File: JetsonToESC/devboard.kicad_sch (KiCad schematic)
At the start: 9 parts, among them U1 ESP32-C3_SUPERMINI_TH, U4 MCP23018x-x-SS

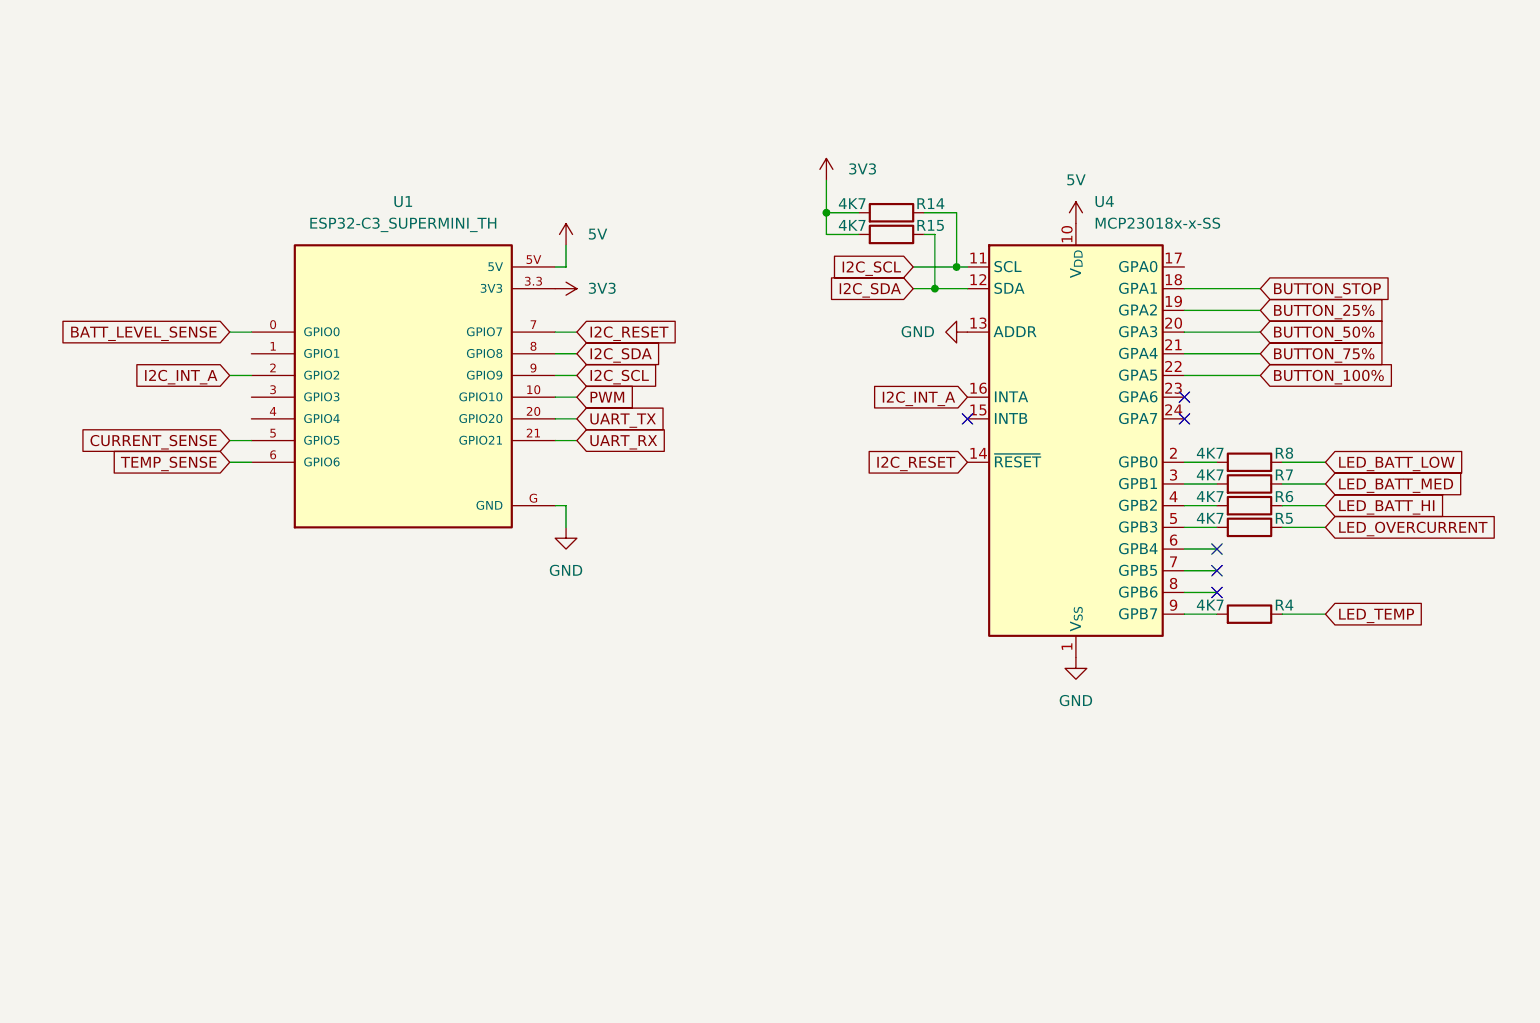
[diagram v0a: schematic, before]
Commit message: Design and routing done
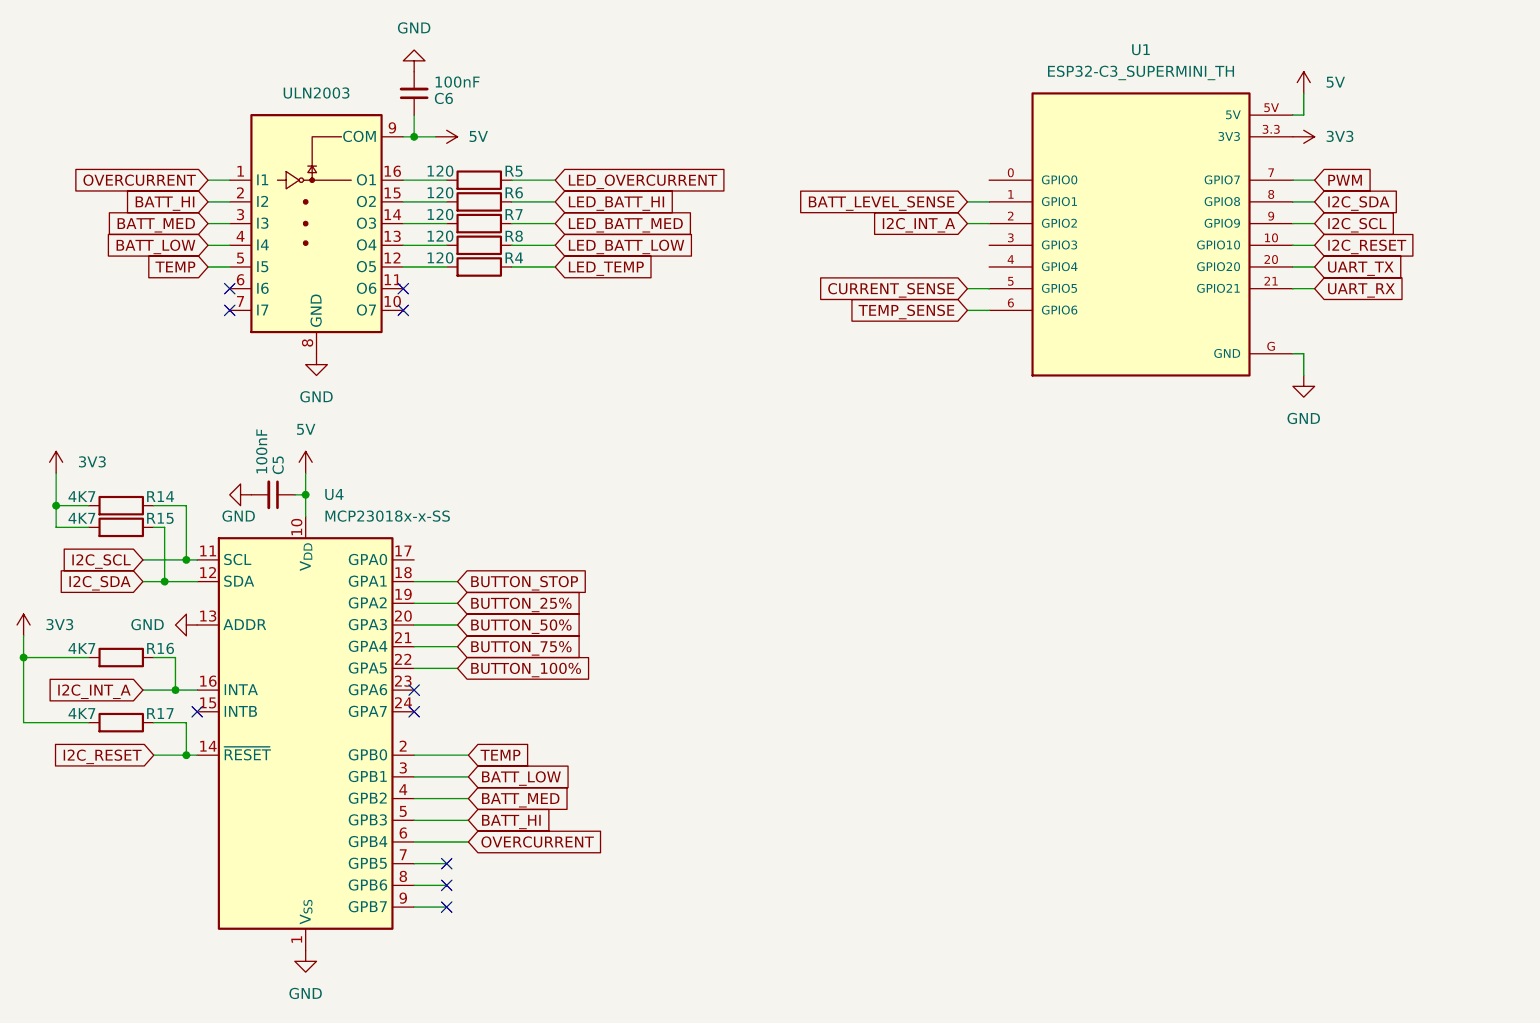
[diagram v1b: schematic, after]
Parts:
- added C5, C6: 100nF, Capacitor_SMD:C_0603_1608Metric, symbol Device:C_Small
- added R16, R17: 4K7, Resistor_SMD:R_0603_1608Metric, symbol Device:R
- added U6: ULN2003, Package_SO:TSSOP-16_4.4x5mm_P0.65mm, symbol Transistor_Array:ULN2003
- R4: value 4K7 -> 120
- R5: renamed from R8; value 4K7 -> 120
- R6: renamed from R7; value 4K7 -> 120
- R7: renamed from R6; value 4K7 -> 120
- R8: renamed from R5; value 4K7 -> 120
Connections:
- net 3V3: now also R16.2, R17.2
- net 5V: now also C5.1, C6.1, U6.9 (COM)
- net BATT_LEVEL_SENSE: now also U1.1 (GPIO1); no longer U1.0 (GPIO0)
- net GND: now also C5.2, C6.2, U6.8 (GND)
- net I2C_INT_A: now also R16.1
- net I2C_RESET: now also U1.10 (GPIO10), R17.1; no longer U1.7 (GPIO7)
- net LED_BATT_HI: now also R6.1; no longer R7.1
- net LED_BATT_LOW: now also R8.1; no longer R5.1
- net LED_BATT_MED: now also R7.1; no longer R6.1
- net LED_OVERCURRENT: now also R5.1; no longer R8.1
- net PWM: now also U1.7 (GPIO7); no longer U1.10 (GPIO10)
- net at R6.2: now also U6.15 (O2); no longer U4.3 (GPB1)
- net at R7.2: now also U6.14 (O3); no longer U4.4 (GPB2)
- net at R5.2: now also U6.16 (O1); no longer U4.2 (GPB0)
- net at R8.2: now also U6.13 (O4); no longer U4.5 (GPB3)
- net OVERCURRENT: now reaches U4.6 (GPB4)
- net OVERCURRENT: now also U6.1 (I1)
- net at U4.9 (GPB7): no longer R4.2
- new net: R4.2, U6.12 (O5)
- new net BATT_HI: U4.5 (GPB3), U6.2 (I2)
- new net BATT_LOW: U4.3 (GPB1), U6.4 (I4)
- new net BATT_MED: U4.4 (GPB2), U6.3 (I3)
- new net TEMP: U4.2 (GPB0), U6.5 (I5)
- no-connect marks 6 -> 10
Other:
- moved on the sheet: R14, R15, R5, R6, R7, R8, U1, U4
